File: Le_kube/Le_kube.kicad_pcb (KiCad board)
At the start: 2 copper layers, 50 x 125 mm, 50 parts, among them J1 Conn_01x06_Male, J2 USB_A, J3 Barrel_Jack_Switch, Q1 IRLB8721PBF, SW1 I/O, SW2 RST, SW3 SW_Push, SW4 SW_Push, SW5 SW_Push, U0 ATmega328PB-AU, U1 LM75A, U2 128x64_OLED, U3 TLC555CDR, U4 ESP8266-01_ESP-01, Y1 Crystal

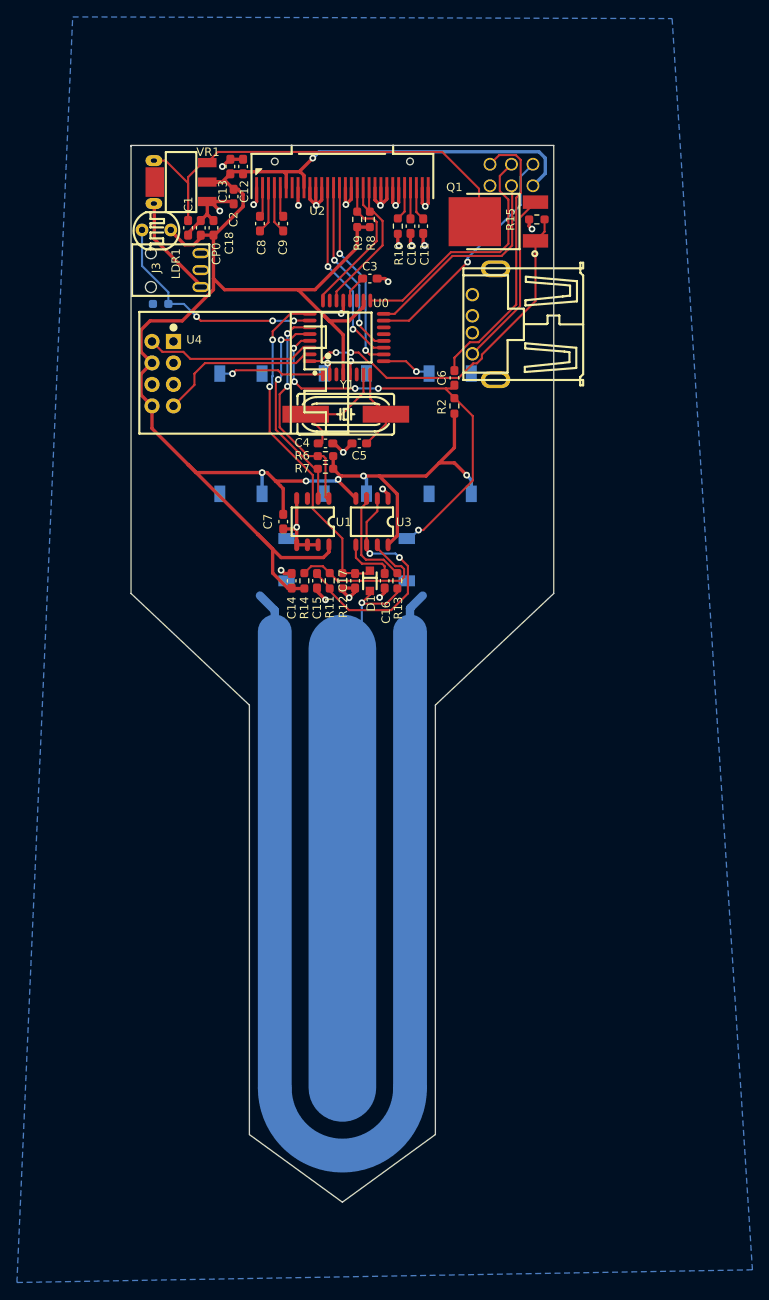
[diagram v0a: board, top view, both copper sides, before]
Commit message: routage done
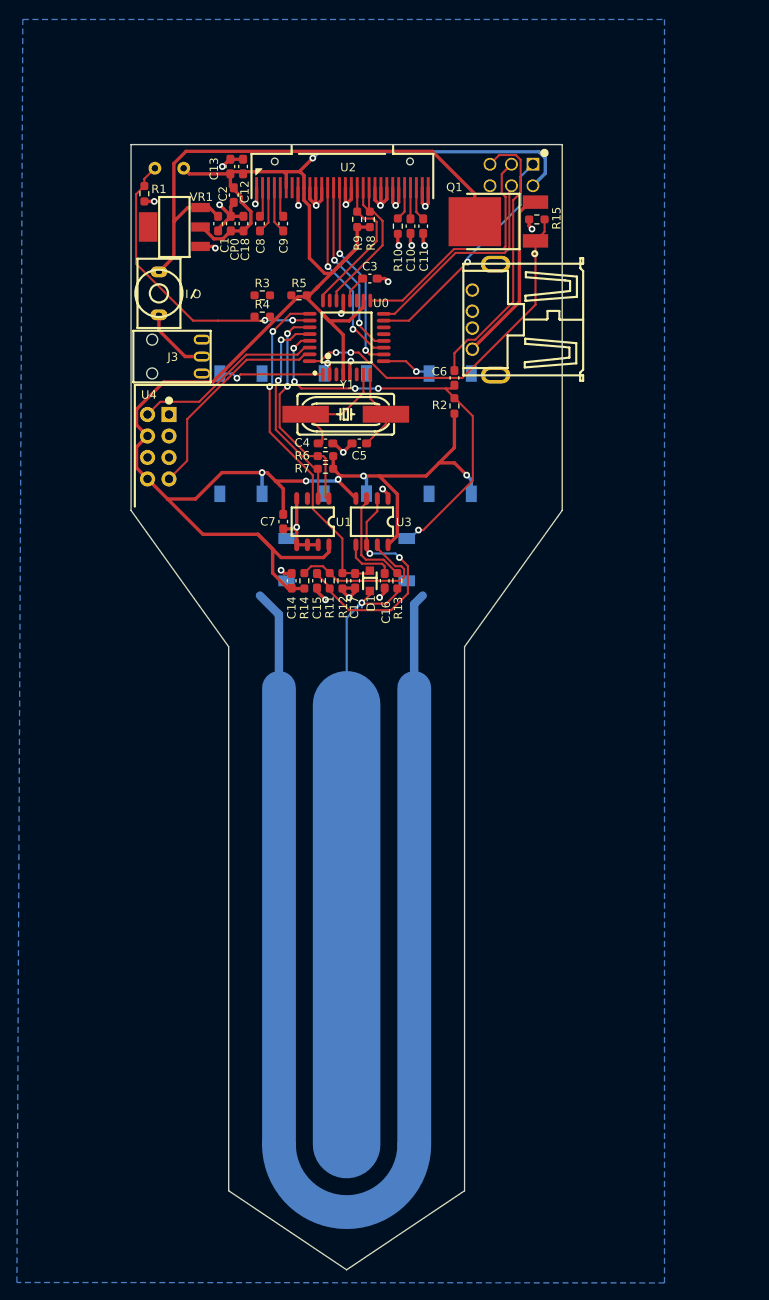
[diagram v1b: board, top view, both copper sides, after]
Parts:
- removed SW1: I/O, Le_kube:SW-TH_L8.0-W5.11-P5.08_TP11SH8CQE
- added I O: I/O, Le_kube:SW-TH_L8.0-W5.11-P5.08_TP11SH8CQE, F.Cu at (78.3, 72.5)
- added R3: 10K, Le_kube:R_0603_1608Metric_Pad0.98x0.95mm_HandSolder, F.Cu at (90.5, 72.7)
- added R4: 10K, Le_kube:R_0603_1608Metric_Pad0.98x0.95mm_HandSolder, F.Cu at (90.5, 75.2)
- added R5: 10K, Le_kube:R_0603_1608Metric_Pad0.98x0.95mm_HandSolder, F.Cu at (94.9, 72.7)
- C19: value PROBE -> GROUND
- LDR1: moved to B.Cu
- R1: moved to F.Cu
- moved R1 13.2 mm to (76.6, 60.7), turned to 90 degrees
- moved J3 10.2 mm to (83.4, 80.0)
- moved U4 8.66 mm to (78.2, 90.6)
- moved LDR1 7.46 mm to (79.5, 57.7), turned to 270 degrees
- moved C19 6.70 mm to (100.5, 117.2)
- moved VR1 5.37 mm to (80.1, 64.7)
- moved C1 3.59 mm to (85.3, 64.2)
- moved C18 3.59 mm to (88.3, 64.2)
- moved CP0 3.59 mm to (86.8, 64.2)
- moved J2 0.54 mm to (116.8, 75.6)
- moved C2 0.17 mm to (87.2, 60.9)
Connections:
- J3 pad 1: +5V -> GND
- J3 pad 2: GND -> +5V
- SW2 pad 2: (no net) -> GND
- SW2 pad 4: GND -> (no net)
- SW3 pad 2: (no net) -> +3V3
- SW3 pad 4: +3V3 -> (no net)
- SW4 pad 2: (no net) -> +3V3
- SW4 pad 4: +3V3 -> (no net)
- SW5 pad 2: (no net) -> +3V3
- SW5 pad 4: +3V3 -> (no net)
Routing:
- net Net-(C19-Pad2): track 64.4 -> 40.0 mm
- net +3V3: track 248.3 -> 258.9 mm
- net Net-(LDR1-Pad1): track 27.6 -> 35.6 mm, vias 3 -> 2
- net /ESP_RX: track 19.4 -> 25.6 mm
- net Net-(C1-Pad2): track 55.4 -> 61.5 mm
- net +5V: track 12.4 -> 8.22 mm
- net /ESP_TX: track 20.1 -> 22.5 mm
- net GND: track 143.1 -> 142.9 mm, vias 23 -> 25
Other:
- board size 50 x 125 mm -> 51 x 133.1 mm
- rule trace_min: 0.2 -> 0.127
- rule via_min_drill: 0.3 -> 0.2
- board text added: "DWN"
- board text added: "Le_Kube"
- board text added: "RST"
- board text added: "SLCT"
- board text added: "UP"
